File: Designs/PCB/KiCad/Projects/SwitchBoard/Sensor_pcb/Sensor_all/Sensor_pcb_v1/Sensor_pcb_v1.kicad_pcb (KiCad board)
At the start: 2 copper layers, 29 parts, among them J1 Header 3x2, J2 Prog Hdr, J3 Solar_input, J4 SWD, J5 Battery_input, SW1 SW_Push, SW2 SW_Push, U1 APK2112.K-3.3, U2 STM32, U3 LoRa, U4 BME_280, U5 Select_IN, Y1 32.768K, Y2 8Mhz

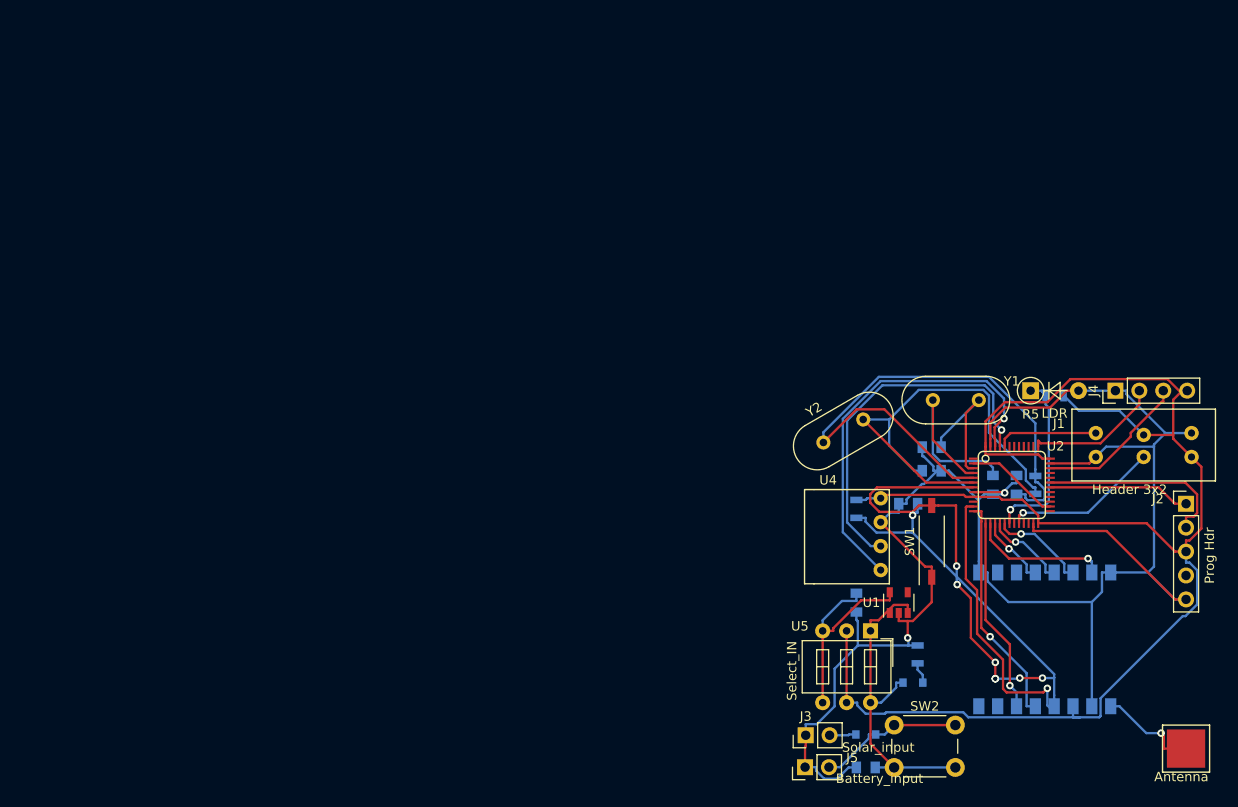
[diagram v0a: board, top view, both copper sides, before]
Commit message: update
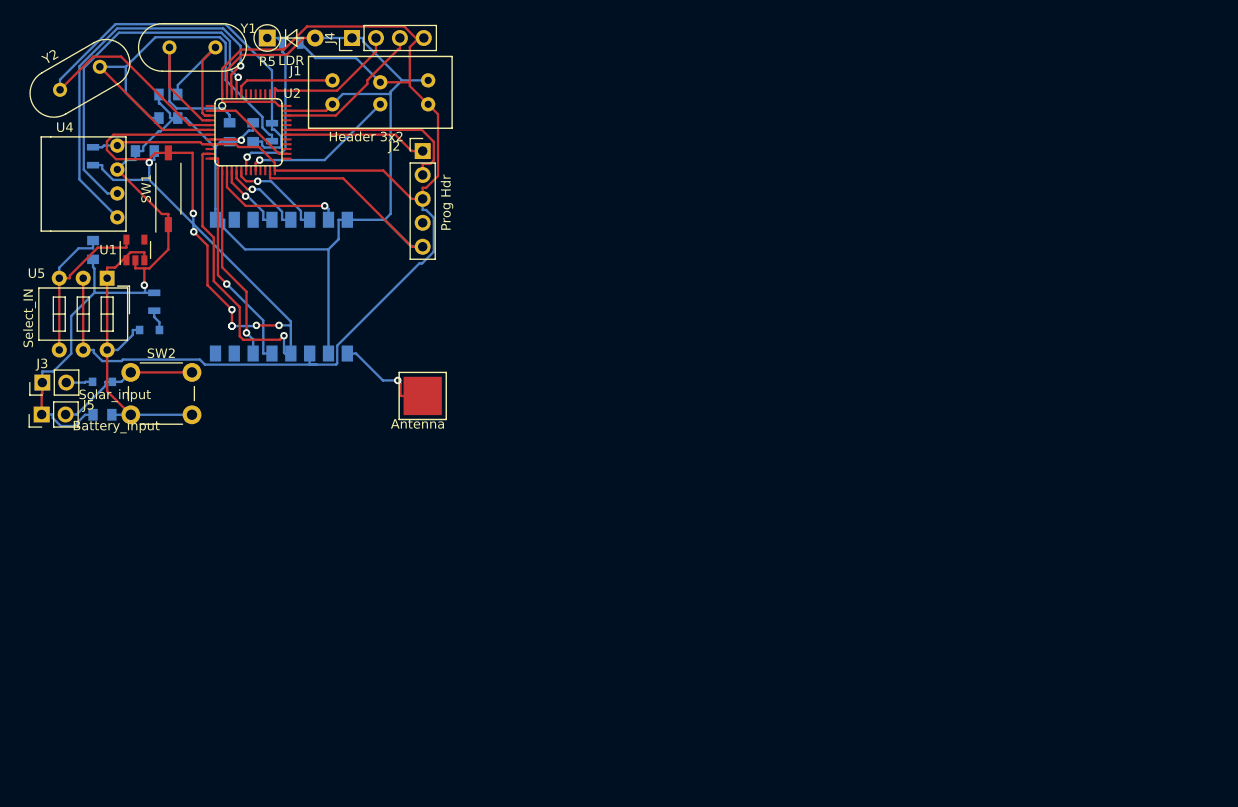
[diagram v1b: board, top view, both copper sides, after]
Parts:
- moved R4 89.3 mm to (52.0, 21.1)
- moved AE1 89.3 mm to (66.0, 58.6)
- moved J2 89.3 mm to (66.0, 32.6)
- moved J3 89.3 mm to (25.6, 57.1)
- moved SW2 89.3 mm to (35.0, 56.1)
- moved C1 89.3 mm to (36.5, 32.6)
- moved C2 89.3 mm to (39.0, 26.6)
- moved C3 89.3 mm to (45.5, 30.6)
- moved C4 89.3 mm to (48.0, 30.6)
- moved C5 89.3 mm to (39.0, 29.1)
- moved C6 89.3 mm to (32.0, 60.6)
- moved C7 89.3 mm to (31.0, 43.1)
- moved D1 89.3 mm to (37.0, 51.6)
- moved D2 89.3 mm to (32.0, 57.1)
- moved J1 89.3 mm to (61.5, 25.1)
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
